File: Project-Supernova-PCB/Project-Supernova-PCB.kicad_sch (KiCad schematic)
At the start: 34 parts, among them J1 Conn_01x04, J103 Screw_Terminal_01x02, J104 Conn_01x02, J105 Conn_01x02, J106 Screw_Terminal_01x02, J107 Conn_Coaxial, J108 Conn_01x04, J109 Screw_Terminal_01x02, J2 Screw_Terminal_01x02, J3 Conn_01x02, J6 100k_Thermistor, J7 100k_Thermistor, Q101 Si1470DH, SW1 SW_SPDT, SW2 SW_SPDT, U1 S09, U101 BMP280-Module, U102 GY-NEO6MV2-Module, U103 LoRa-E5, U2 ESP32-Module-30Pin, U3 LM335D

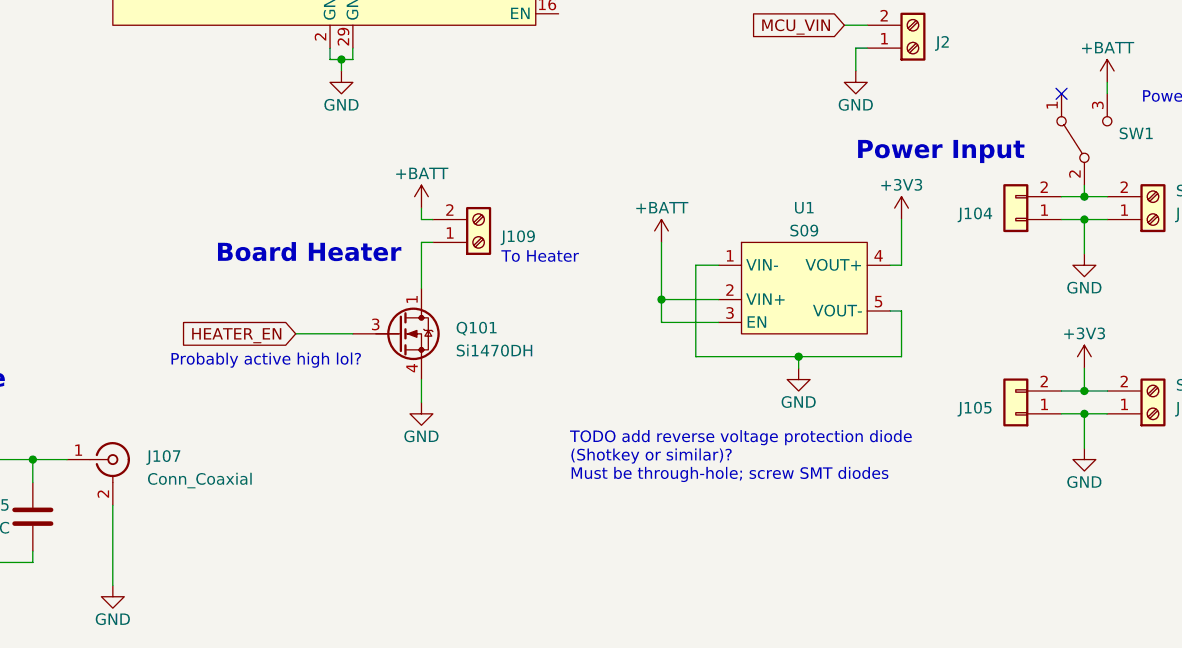
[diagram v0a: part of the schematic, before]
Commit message: More work
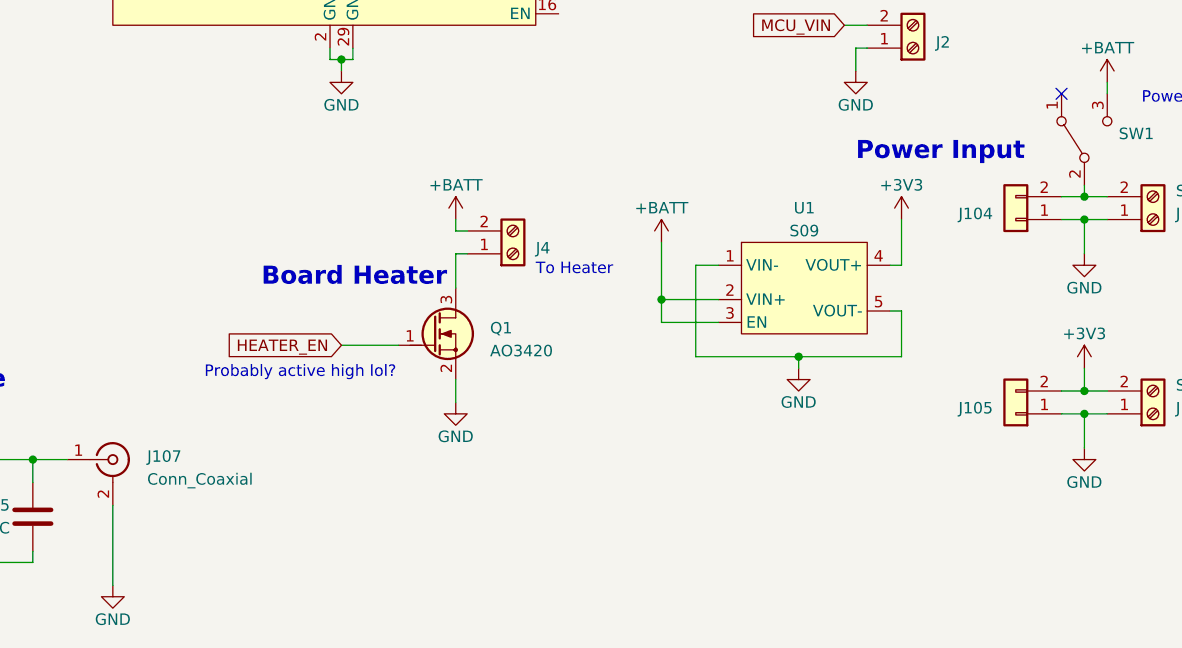
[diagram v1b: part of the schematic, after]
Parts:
- removed J109: Screw_Terminal_01x02, TerminalBlock:TerminalBlock_bornier-2_P5.08mm, symbol Connector:Screw_Terminal_01x02
- removed Q101: Si1470DH, Package_TO_SOT_SMD:SOT-363_SC-70-6, symbol Transistor_FET:Si1442DH
- added J4: Screw_Terminal_01x02, TerminalBlock:TerminalBlock_bornier-2_P5.08mm, symbol Connector:Screw_Terminal_01x02
- added Q1: AO3420, Package_TO_SOT_SMD:SOT-23, symbol PCM_Transistor_MOSFET_AKL:AO3420
- J3: footprint (none) -> Connector_PinHeader_2.54mm:PinHeader_1x02_P2.54mm_Vertical
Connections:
- net +BATT: now also J4.2 (Pin_2)
- net GND: now also Q1.2 (S)
- net HEATER_EN: now also Q1.1 (G)
- new net: J4.1 (Pin_1), Q1.3 (D)
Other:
- note removed: "TODO add reverse voltage protection diode (Shotkey or similar)? Must be through-hole; screw SMT diodes"
